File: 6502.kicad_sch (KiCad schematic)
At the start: 7 parts, among them U1 W65C02, U2 W65C22, U3 28C256, U4 62256, U5 W65C22

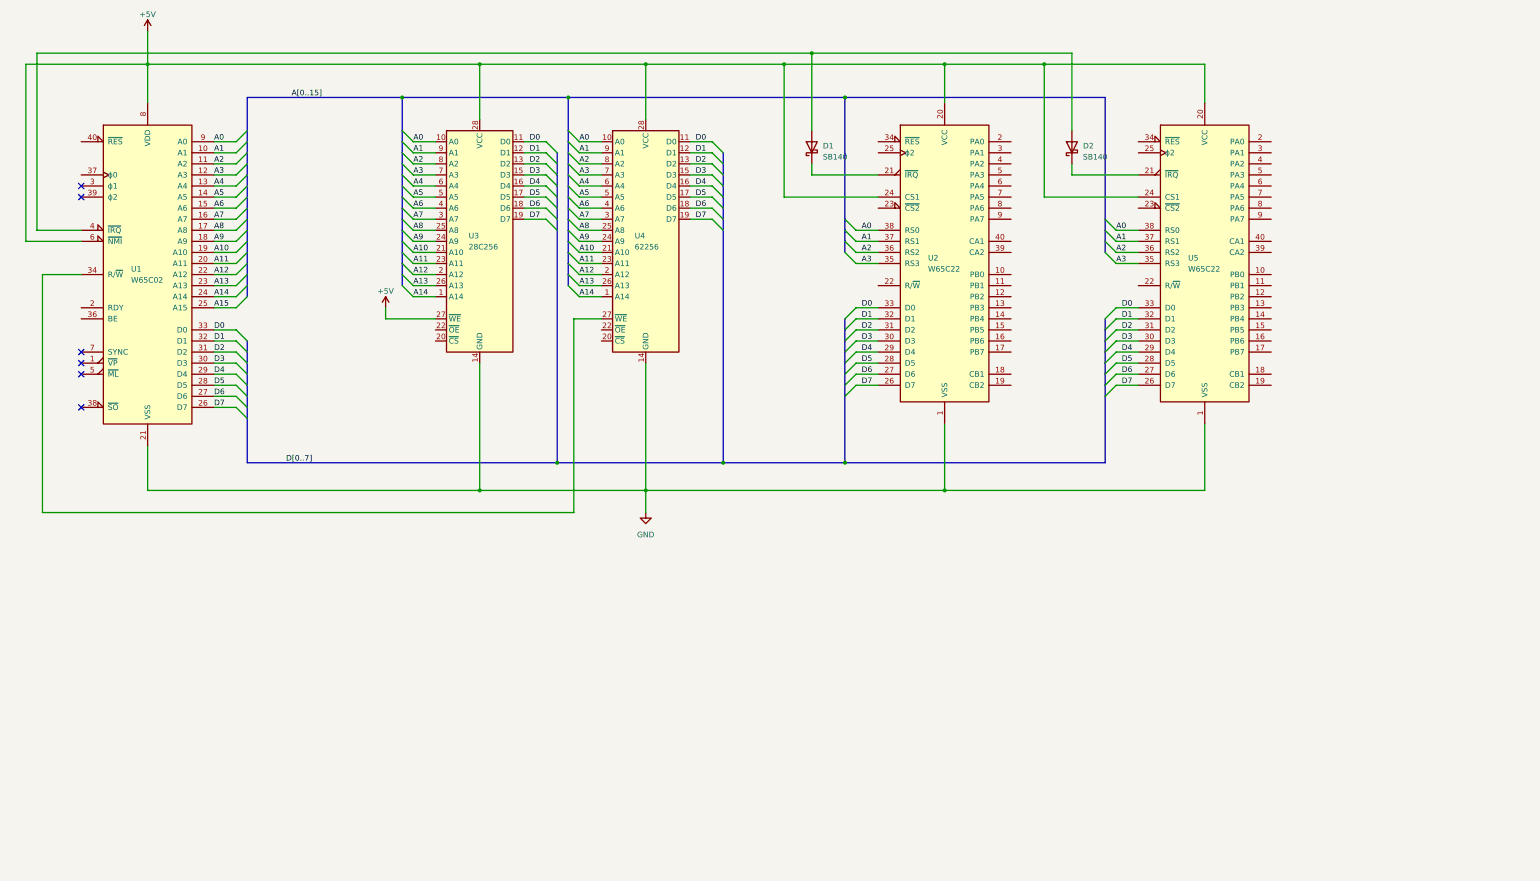
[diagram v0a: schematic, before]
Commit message: Updated schematic design files
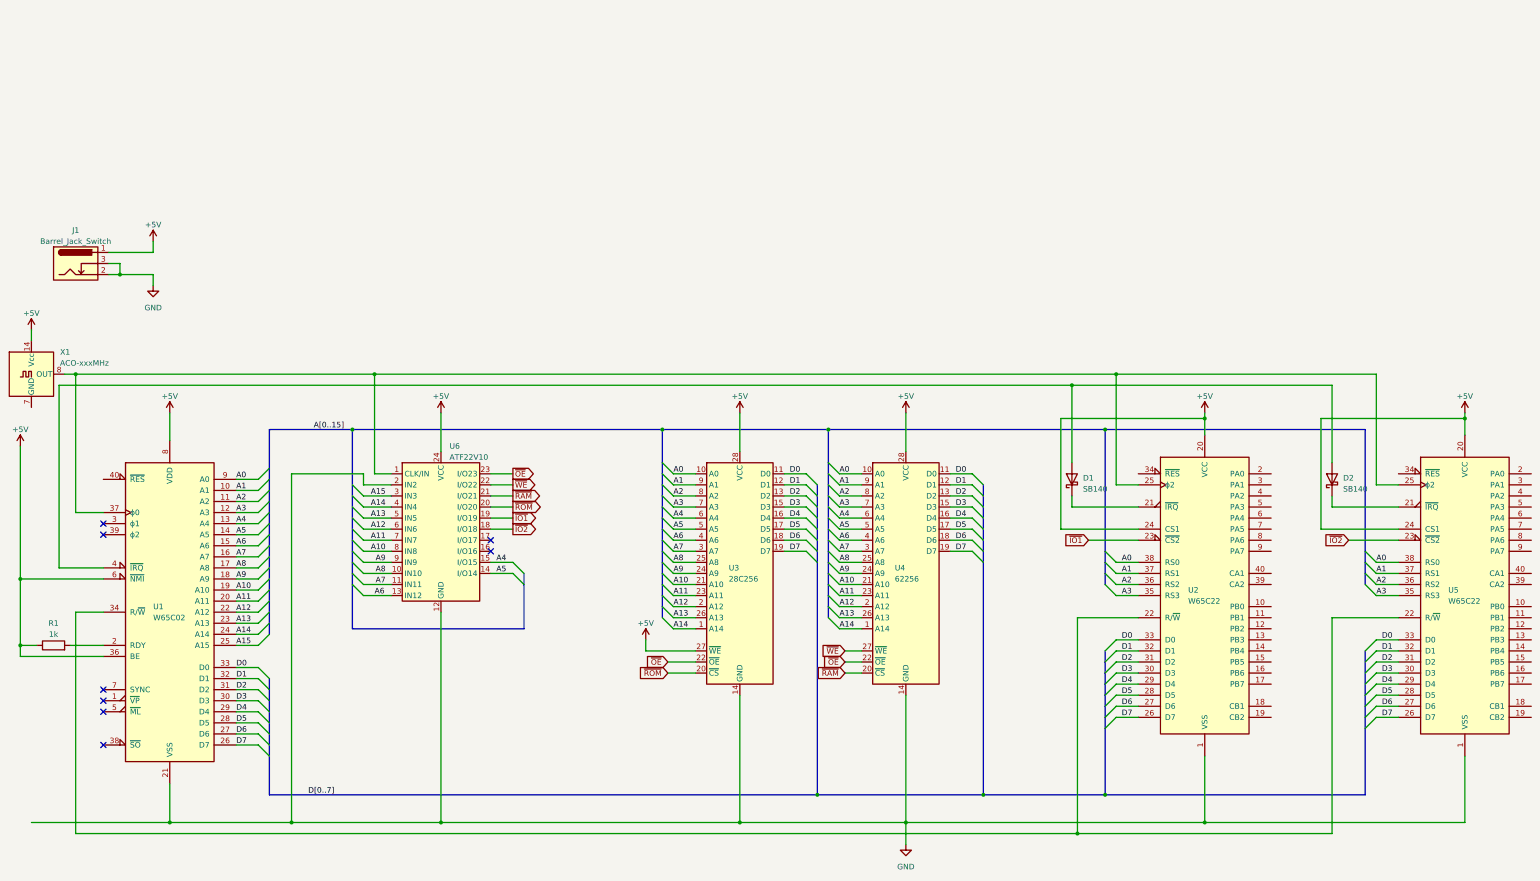
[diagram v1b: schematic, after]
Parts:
- added J1: Barrel_Jack_Switch, Connector_BarrelJack:BarrelJack_Wuerth_6941xx301002, symbol Connector:Barrel_Jack_Switch
- added R1: 1k, Resistor_THT:R_Axial_DIN0207_L6.3mm_D2.5mm_P7.62mm_Horizontal, symbol Device:R
- added U6: ATF22V10, Package_DIP:DIP-24_W7.62mm_Socket, symbol ATF:ATF22V10
- added X1: ACO-xxxMHz, Oscillator:Oscillator_DIP-14, symbol Oscillator:ACO-xxxMHz
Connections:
- net +5V: now also U1.36 (BE), J1.1, R1.1, U6.24 (VCC), X1.14 (Vcc)
- net A10: now also U6.8 (IN8)
- net A11: now also U6.7 (IN7)
- net A12: now also U6.6 (IN6)
- net A13: now also U6.5 (IN5)
- net A14: now also U6.4 (IN4)
- net A15: now also U6.3 (IN3)
- net A4: now also U6.15 (I/O15)
- net A5: now also U6.14 (I/O14)
- net A6: now also U6.13 (IN12)
- net A7: now also U6.11 (IN11)
- net A8: now also U6.10 (IN10)
- net A9: now also U6.9 (IN9)
- net GND: now also J1.2, J1.3, U6.12 (GND), U6.2 (IN2)
- net at U5.22 (R/~{W}): now also U1.34 (R/~{W}), U2.22 (R/~{W})
- net ~{IO2}: now reaches U5.23 (~{CS2})
- net ~{IO2}: now also U6.18 (I/O18)
- net at U5.25 (ϕ2): now also U1.37 (ϕ0), U2.25 (ϕ2), U6.1 (CLK/IN), X1.8 (OUT)
- net ~{ROM}: now reaches U3.20 (~{CS})
- net ~{ROM}: now also U6.20 (I/O20)
- net ~{OE}: now reaches U3.22 (~{OE})
- net ~{OE}: now also U4.22 (~{OE}), U6.23 (I/O23)
- net ~{IO1}: now reaches U2.23 (~{CS2})
- net ~{IO1}: now also U6.19 (I/O19)
- net at U1.2 (RDY): now also R1.2
- net ~{WE}: now reaches U4.27 (~{WE})
- net ~{WE}: now also U6.22 (I/O22); no longer U1.34 (R/~{W})
- net ~{RAM}: now reaches U4.20 (~{CS})
- net ~{RAM}: now also U6.21 (I/O21)
- no-connect marks 6 -> 8
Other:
- moved on the sheet: D1, D2, U1, U2, U3, U4, U5
